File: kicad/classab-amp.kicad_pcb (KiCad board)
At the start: 2 copper layers, 84.5 x 82.5 mm, 67 parts, among them J1 SPEAKER, J3 INPUT, Q1 2N5551, Q10 IRFP9240, Q11 2N5551, Q12 2N5551, Q15 2N5551, Q16 2N5401, Q2 2N5551, Q3 2N5401, Q4 2N5401, Q6 BD140, Q7 BD139, Q8 BD139, Q9 IRFP240

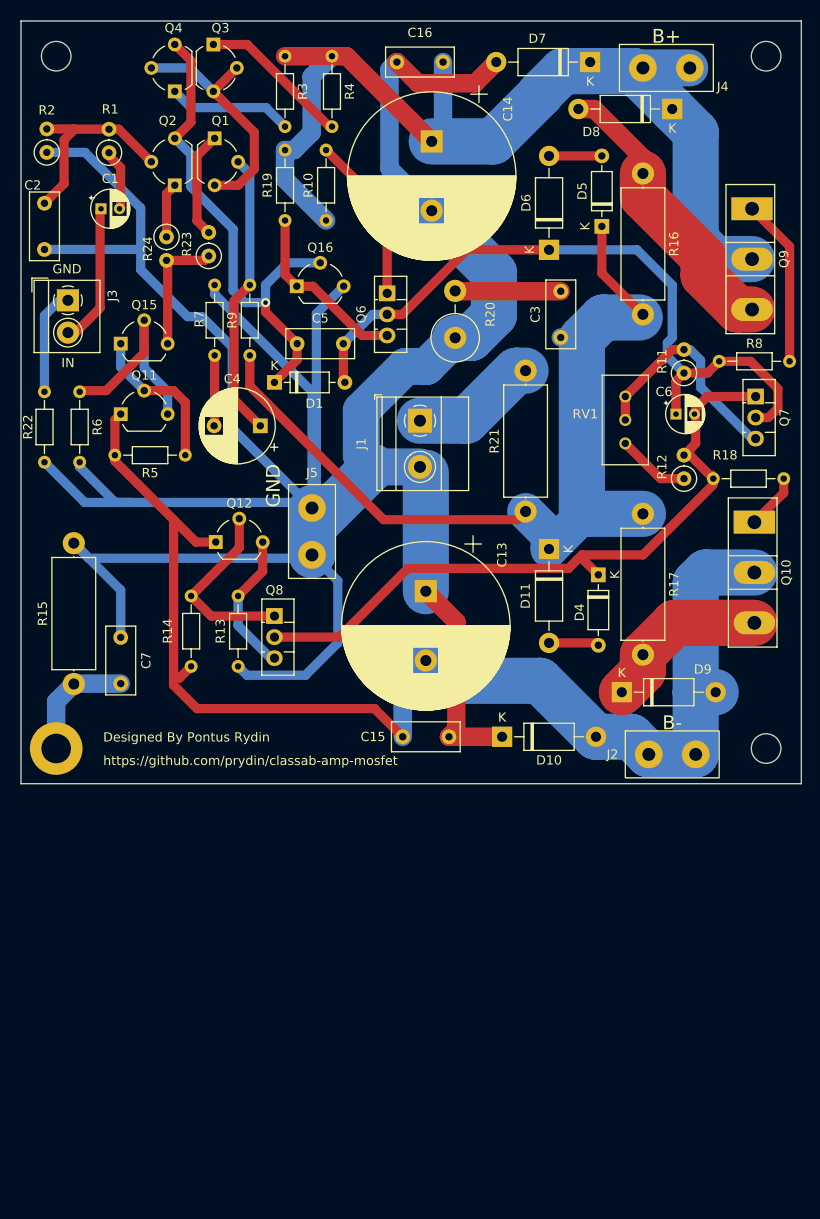
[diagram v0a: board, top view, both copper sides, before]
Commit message: Pre re-layout
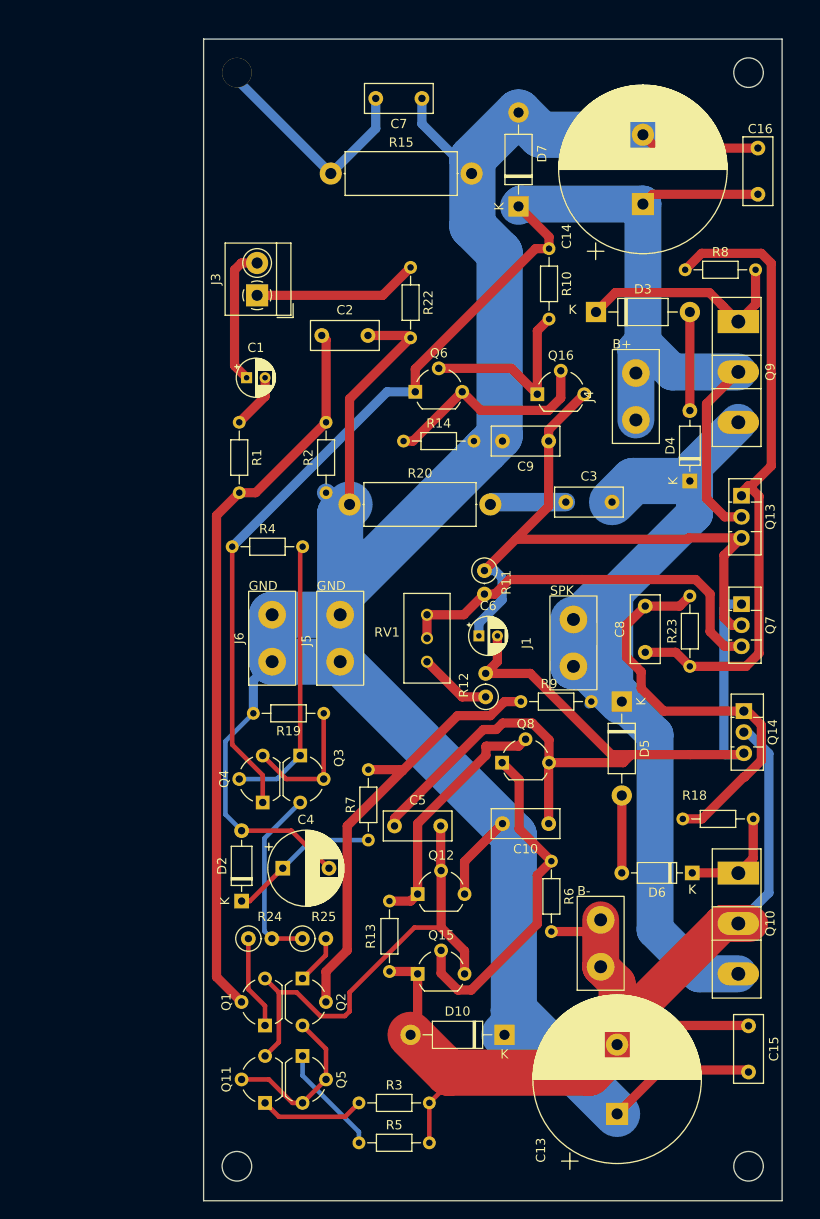
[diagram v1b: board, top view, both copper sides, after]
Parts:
- removed ?: , 
- removed D1: 1N4148, Diode_THT:D_DO-35_SOD27_P7.62mm_Horizontal
- removed D11: 1N5919, Diode_THT:D_DO-41_SOD81_P10.16mm_Horizontal
- removed D8, D9: 1N4004, Diode_THT:D_DO-41_SOD81_P10.16mm_Horizontal
- removed R16, R17: 0.33, Resistor_THT:R_Axial_DIN0414_L11.9mm_D4.5mm_P15.24mm_Horizontal
- removed R21: 10, Resistor_THT:R_Axial_DIN0414_L11.9mm_D4.5mm_P15.24mm_Horizontal
- removed the REF** at (196.8, 34.3)
- removed the REF** at (273.7, 34.3)
- added C10: 68p, Capacitor_THT:C_Rect_L7.2mm_W3.0mm_P5.00mm_FKS2_FKP2_MKS2_MKP2, F.Cu at (250.2, 117.3)
- added C8: 220n, Capacitor_THT:C_Rect_L7.2mm_W3.0mm_P5.00mm_FKS2_FKP2_MKS2_MKP2, F.Cu at (260.6, 98.8)
- added C9: 68p, Capacitor_THT:C_Rect_L7.2mm_W3.0mm_P5.00mm_FKS2_FKP2_MKS2_MKP2, F.Cu at (250.2, 75.9)
- added D2: 1N4148, Diode_THT:D_DO-35_SOD27_P7.62mm_Horizontal, F.Cu at (216.9, 125.7)
- added D3: 1N5919, Diode_THT:D_DO-41_SOD81_P10.16mm_Horizontal, F.Cu at (255.3, 62.0)
- added J6: ~, footprints:Spade Connector, F.Cu at (215.1, 97.3)
- added Q13: BD139, Package_TO_SOT_THT:TO-126-3_Vertical, F.Cu at (271.0, 81.9)
- added Q14: BD140, Package_TO_SOT_THT:TO-126-3_Vertical, F.Cu at (271.3, 105.2)
- added Q5: 2N5551, Package_TO_SOT_THT:TO-92_Wide, F.Cu at (223.5, 142.5)
- added R25: 100, Resistor_THT:R_Axial_DIN0207_L6.3mm_D2.5mm_P2.54mm_Vertical, F.Cu at (223.5, 129.8)
- added REF**: MountingHole_3.2mm_M3, MountingHole:MountingHole_3.2mm_M3, F.Cu at (271.8, 36.1)
- added REF**: MountingHole_3.2mm_M3, MountingHole:MountingHole_3.2mm_M3, F.Cu at (216.4, 36.1)
- added REF**: MountingHole_3.2mm_M3, MountingHole:MountingHole_3.2mm_M3, F.Cu at (216.4, 154.4)
- C5: value 100p -> 33p
- D5: value 1N4148 -> 1N5919; footprint Diode_THT:D_DO-35_SOD27_P7.62mm_Horizontal -> Diode_THT:D_DO-41_SOD81_P10.16mm_Horizontal
- D6: value 1N5919 -> 1N4148; footprint Diode_THT:D_DO-41_SOD81_P10.16mm_Horizontal -> Diode_THT:D_DO-35_SOD27_P7.62mm_Horizontal
- J1: value SPEAKER -> ~; footprint TerminalBlock_Phoenix:TerminalBlock_Phoenix_MKDS-1,5-2_1x02_P5.00mm_Horizontal -> footprints:Spade Connector
- Q1, Q2: value 2N5551 -> 2N5401
- Q6: value BD140 -> 2N5401; footprint Package_TO_SOT_THT:TO-126-3_Vertical -> Package_TO_SOT_THT:TO-92_Wide
- Q8: value BD139 -> 2N5551; footprint Package_TO_SOT_THT:TO-126-3_Vertical -> Package_TO_SOT_THT:TO-92_Wide
- R1, R2: footprint Resistor_THT:R_Axial_DIN0207_L6.3mm_D2.5mm_P2.54mm_Vertical -> Resistor_THT:R_Axial_DIN0204_L3.6mm_D1.6mm_P7.62mm_Horizontal
- R10: value 100 -> 47
- R11: value 4.7k -> 10k
- R12: value 330 -> 680
- R13: value 10k -> 1k
- R14: value 100 -> 10k
- R18, R8: value 330 -> 47
- R19: value 1k -> 10k
- R20: footprint Resistor_THT:R_Axial_DIN0516_L15.5mm_D5.0mm_P5.08mm_Vertical -> Resistor_THT:R_Axial_DIN0414_L11.9mm_D4.5mm_P15.24mm_Horizontal
- R23: value 100 -> 680; footprint Resistor_THT:R_Axial_DIN0207_L6.3mm_D2.5mm_P2.54mm_Vertical -> Resistor_THT:R_Axial_DIN0204_L3.6mm_D1.6mm_P7.62mm_Horizontal
- R4: value 470 -> 1k
- R6: value 4.7k -> 22
- moved R3 113.6 mm to (229.6, 147.6), turned to 0 degrees
- moved Q1 96.2 mm to (219.4, 139.2), turned to 90 degrees
- moved Q2 87.0 mm to (223.5, 134.1), turned to -90 degrees
- moved Q4 77.5 mm to (219.2, 115.1)
- moved Q3 77.5 mm to (223.3, 110.0)
- moved R5 76.8 mm to (229.6, 151.9), turned to 0 degrees
- moved R24 76.5 mm to (217.6, 129.8), turned to 0 degrees
- moved Q11 76.2 mm to (219.5, 147.6), turned to 90 degrees
- moved Q15 75.4 mm to (236.0, 133.6)
- moved R6 72.0 mm to (250.4, 121.4)
- moved D6 69.2 mm to (265.7, 122.7), turned to 180 degrees
- moved R23 68.4 mm to (265.4, 100.3)
- moved C7 66.8 mm to (236.4, 38.9), turned to 180 degrees
- moved R7 62.3 mm to (230.6, 119.1), turned to 90 degrees
- moved R15 61.9 mm to (226.6, 47.0), turned to 0 degrees
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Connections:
- C2 pad 1: Net-(Q2-B) -> Net-(Q1-B)
- C3 pad 1: Net-(D11-K) -> /SPEAKER
- C4 pad 1: Net-(Q1-B) -> Net-(D2-K)
- C4 pad 2: Net-(C4-Pad2) -> PWRGND
- C5 pad 1: Net-(D1-K) -> Net-(Q1-C)
- C5 pad 2: Net-(D1-A) -> Net-(Q14-B)
- C6 pad 1: Net-(D1-A) -> Net-(Q13-B)
- C6 pad 2: Net-(D4-K) -> Net-(Q14-B)
- D4 pad 1: Net-(D4-K) -> /SPEAKER
- D5 pad 1: Net-(D11-K) -> /SPEAKER
- D6 pad 1: Net-(D1-A) -> Net-(D6-K)
- J1 pad 2: PWRGND -> /SPEAKER
- Q1 pad 3: /LTP COM -> Net-(Q1-C)
- Q10 pad 1: Net-(Q10-G) -> Net-(D6-K)
- Q10 pad 3: Net-(D9-K) -> /SPEAKER
- Q11 pad 1: B- -> Net-(Q11-E)
- Q11 pad 3: Net-(Q11-C) -> Net-(Q1-C)
- Q12 pad 1: B- -> Net-(Q12-E)
- Q12 pad 2: Net-(Q12-B) -> Net-(Q1-C)
- Q12 pad 3: Net-(Q12-C) -> PWRGND
- Q15 pad 1: Net-(Q11-B) -> B-
- Q15 pad 2: Net-(Q11-C) -> Net-(Q15-B)
- Q15 pad 3: Net-(Q15-C) -> Net-(Q1-C)
- Q16 pad 2: Net-(D1-K) -> Net-(Q16-B)
- Q16 pad 3: PWRGND -> Net-(Q13-B)
- Q2 pad 1: Net-(Q2-E) -> /LTP COM
- Q2 pad 3: Net-(D1-K) -> Net-(Q11-B)
- Q3 pad 2: /LTP COM -> Net-(Q3-B)
- Q3 pad 3: /LTP COM -> Net-(Q3-C)
- Q4 pad 1: Net-(Q4-E) -> B+
- Q4 pad 2: /LTP COM -> Net-(Q3-E)
- Q4 pad 3: Net-(D1-K) -> Net-(Q3-B)
- Q6 pad 1: Net-(Q6-E) -> B+
- Q6 pad 2: Net-(D1-A) -> Net-(Q16-E)
- Q6 pad 3: Net-(Q16-E) -> Net-(Q16-B)
- Q7 pad 1: Net-(D4-K) -> Net-(Q14-B)
- Q7 pad 2: Net-(D1-A) -> Net-(Q13-B)
- Q8 pad 1: Net-(Q12-B) -> Net-(Q15-B)
- Q8 pad 2: Net-(D4-K) -> Net-(Q12-E)
- Q8 pad 3: Net-(Q12-C) -> Net-(Q14-B)
- Q9 pad 3: Net-(D8-A) -> /SPEAKER
- R1 pad 2: Net-(Q2-B) -> Net-(Q1-B)
- R10 pad 2: Net-(Q6-E) -> Net-(Q16-E)
- R11 pad 1: Net-(D1-A) -> Net-(Q13-B)
- R12 pad 2: Net-(D4-K) -> Net-(Q14-B)
- R13 pad 1: Net-(Q12-C) -> Net-(Q12-E)
- R13 pad 2: PWRGND -> B-
- R14 pad 1: Net-(Q12-B) -> Net-(Q16-B)
- R14 pad 2: B- -> PWRGND
- R18 pad 1: Net-(D4-K) -> Net-(Q14-E)
- R18 pad 2: Net-(Q10-G) -> Net-(D6-K)
- R19 pad 1: B+ -> Net-(Q3-B)
- R19 pad 2: Net-(Q16-E) -> PWRGND
- R2 pad 2: Net-(Q2-B) -> Net-(Q1-B)
- R23 pad 1: Net-(Q15-C) -> Net-(Q13-E)
- R23 pad 2: Net-(Q1-E) -> Net-(Q14-E)
- R24 pad 1: Net-(Q2-E) -> Net-(Q1-E)
- R24 pad 2: Net-(Q15-C) -> Net-(Q3-C)
- R3 pad 1: B+ -> Net-(Q11-E)
- R3 pad 2: Net-(Q4-E) -> B-
- R5 pad 1: Net-(Q11-B) -> Net-(Q5-E)
- R6 pad 1: Net-(Q11-C) -> Net-(Q15-B)
- R6 pad 2: PWRGND -> B-
- R7 pad 1: PWRGND -> Net-(D2-K)
- R7 pad 2: Net-(C4-Pad2) -> Net-(Q2-B)
- R8 pad 1: Net-(D1-A) -> Net-(Q13-E)
- R9 pad 1: Net-(Q1-B) -> Net-(Q2-B)
- R9 pad 2: Net-(D11-K) -> /SPEAKER
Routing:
- net Net-(Q14-B): track 0.00 -> 96.6 mm
- net Net-(D11-K): track 96.3 -> 0.00 mm
- net /SPEAKER: track 13.7 -> 100.5 mm
- net Net-(D1-A): track 77.4 -> 0.00 mm
- net Net-(D4-K): track 75.3 -> 0.00 mm
- net Net-(Q13-E): track 0.00 -> 70.6 mm
- net Net-(Q13-B): track 0.00 -> 69.3 mm
- net PWRGND: track 347.1 -> 290.6 mm
- net B+: track 109.3 -> 165.6 mm
- net Net-(D1-K): track 54.6 -> 0.00 mm, vias 1 -> 0
- net Net-(Q1-C): track 0.00 -> 50.7 mm
- net Net-(Q1-B): track 31.0 -> 79.4 mm
- net Net-(Q14-E): track 0.00 -> 45.3 mm
- net Net-(Q15-B): track 0.00 -> 36.9 mm
- net Net-(D8-A): track 31.4 -> 0.00 mm
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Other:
- board size 84.5 x 82.5 mm -> 62.6 x 125.7 mm
- board text added: "SPK"
- board text removed: "Designed By Pontus Rydin"
- board text removed: "IN"
- board text removed: "https://github.com/prydin/classab-amp-mosfet"
